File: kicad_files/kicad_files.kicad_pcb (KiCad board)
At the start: 2 copper layers, 150 x 100 mm, 64 parts, among them J1 Battery Connection, J2 Servo Connection, J3 DC Motor Connection, J4 Washout Ultrasonic Sensor Con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, J5 Water Sensor Connection, J6 Servo Connection, J7 Larvicide Level Ultrasonic Se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, Q1 FS8205A, Q2 NPN, Q3 NMOS, Q4 NMOS, Q5 NPN, Q7 NMOS, U1 BQ27441DRZR-G1A, U2 DW01A, U3 TPS61023DRLR, U4 LM311, U5 LMC555CMMX_NOPB, U6 LMC555CMMX_NOPB

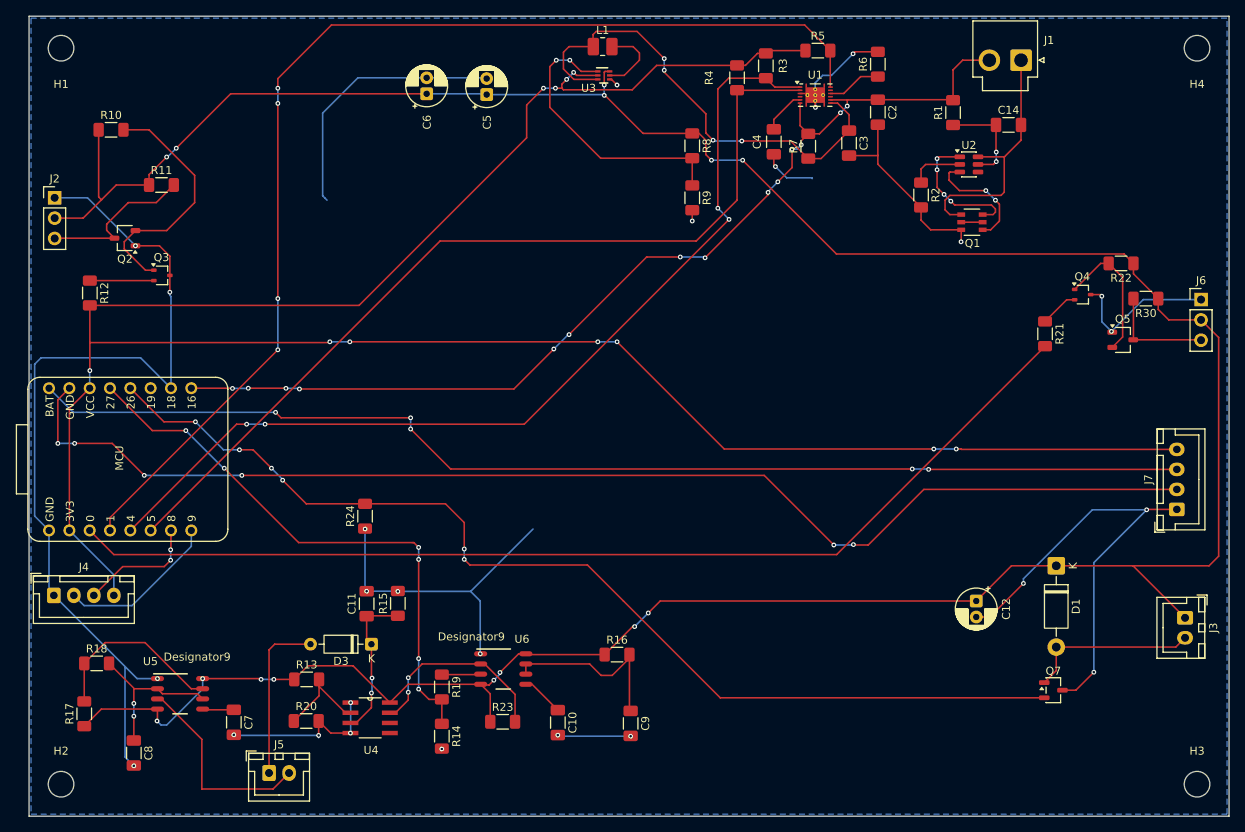
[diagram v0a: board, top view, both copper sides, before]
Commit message: Second pass routing and floorplan
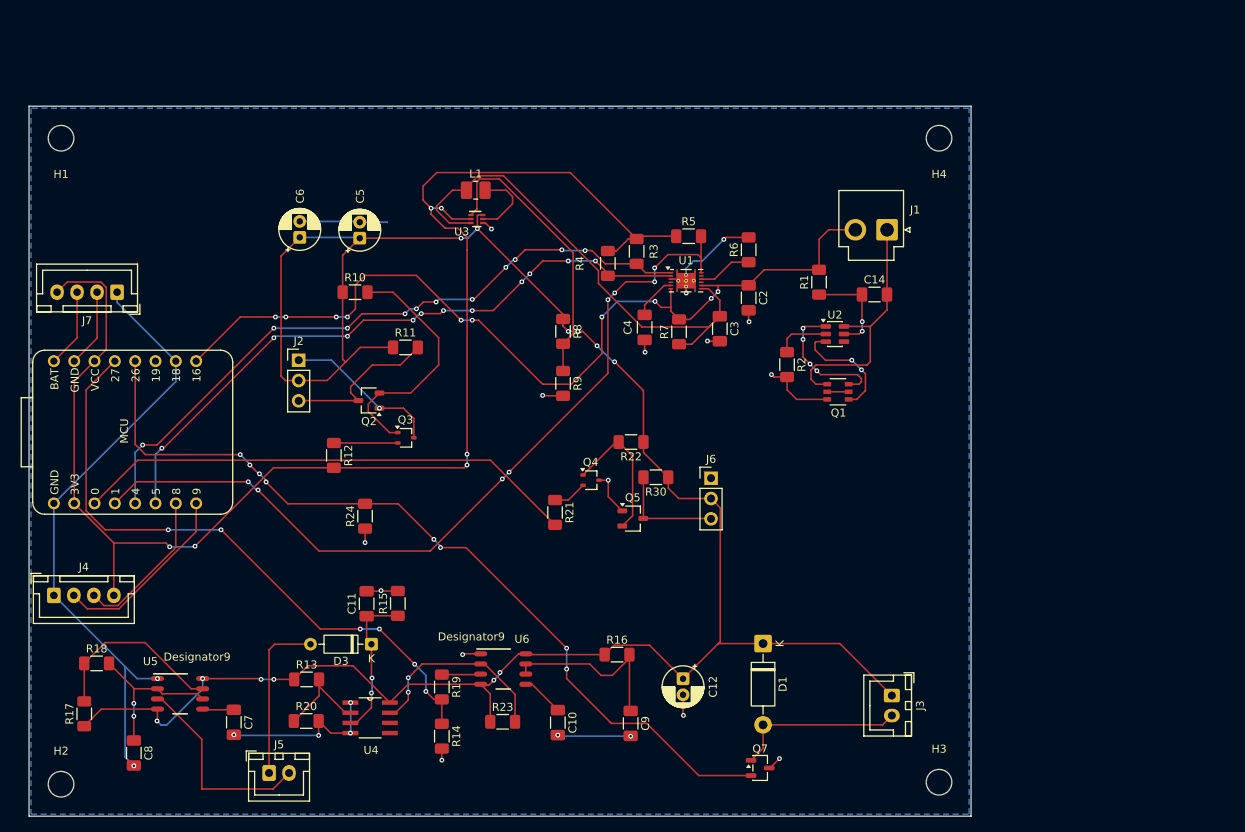
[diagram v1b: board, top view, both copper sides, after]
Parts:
- moved J7 135.2 mm to (111.0, 84.5), turned to 180 degrees
- moved Q4 65.7 mm to (170.2, 108.0)
- moved J6 65.2 mm to (185.2, 107.8)
- moved Q5 65.2 mm to (175.5, 112.8)
- moved R21 65.2 mm to (165.8, 112.0)
- moved R22 65.2 mm to (175.2, 103.2)
- moved R30 65.2 mm to (178.3, 107.6)
- moved C12 37.9 mm to (181.8, 132.8)
- moved Q7 37.9 mm to (191.4, 144.0)
- moved D1 37.9 mm to (191.8, 128.4)
- moved J3 37.9 mm to (207.8, 134.9)
- moved R11 36.6 mm to (147.1, 91.4)
- moved Q2 36.6 mm to (142.5, 98.0)
- moved Q3 36.6 mm to (147.1, 102.7)
- moved R10 36.6 mm to (140.8, 84.5)
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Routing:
- net GND: track 349.7 -> 197.2 mm, vias 26 -> 24
- net /MCU/larvLevelSonarEcho: track 155.6 -> 9.80 mm, vias 6 -> 0
- net /MCU/larvLevelSonarTrig: track 146.0 -> 9.81 mm, vias 5 -> 0
- net /Dispensing Unit/5V: track 380.3 -> 268.9 mm, vias 14 -> 12
- net /MCU/3V3: track 292.1 -> 181.7 mm, vias 11 -> 6
- net /Dispensing Unit/MCU PWM Dispense: track 131.5 -> 63.1 mm
- net /MCU/batteryLevTrigPin: track 142.9 -> 104.5 mm, vias 4 -> 8
- net /MCU/batteryLevDataPin: track 119.1 -> 85.0 mm, vias 4 -> 11
- net /MCU/batteryLevClkPin: track 112.0 -> 81.5 mm, vias 0 -> 11
- net /Dispensing Unit/MCU Motor 1: track 133.0 -> 107.1 mm, vias 6 -> 8
- net /MCU/Bat+: track 127.9 -> 114.3 mm, vias 14 -> 10
- net /MCU/washoutIn: track 71.0 -> 78.6 mm
- net /MCU/washoutSonarTrig: track 15.2 -> 19.3 mm, vias 2 -> 0
- net Net-(U1-SRN): track 60.0 -> 63.3 mm, vias 4 -> 0
- net /MCU/washoutSonarEcho: track 20.3 -> 23.5 mm
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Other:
- board size 150 x 100 mm -> 117.8 x 88.8 mm
